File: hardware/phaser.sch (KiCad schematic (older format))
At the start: 38 parts, among them IC1 STM32F042K4U6, IC2 MCP1700, P1 CONN_01X03, P2 SWD_TC, T1 230/6+6 1VA, U1 VTX-214-003-105

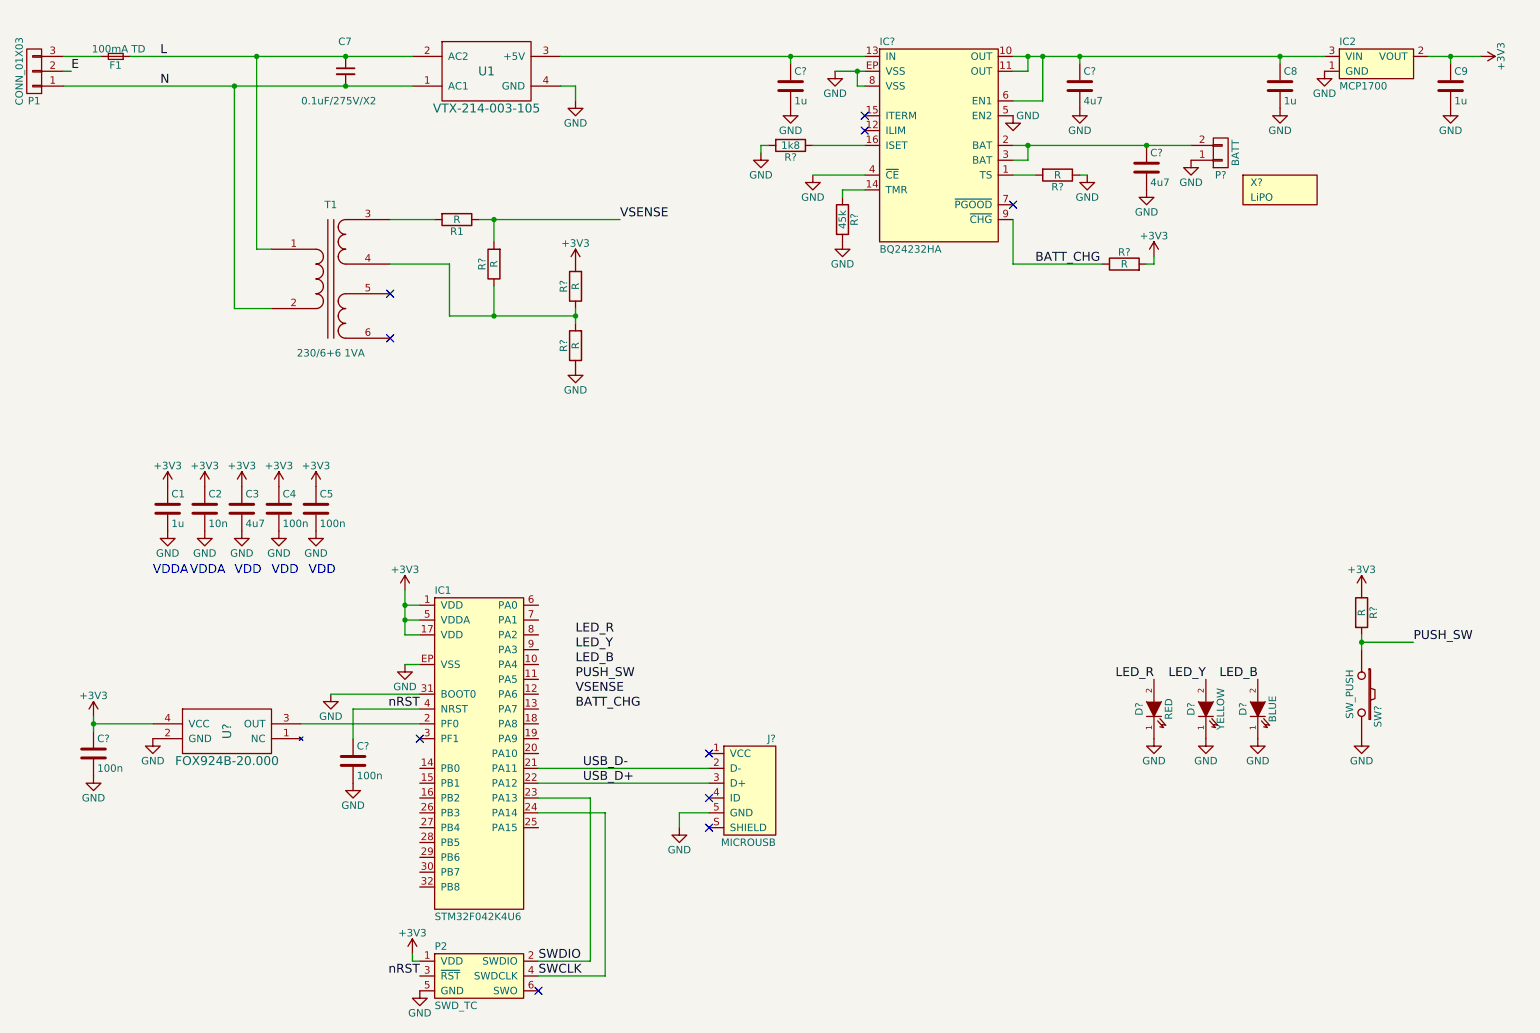
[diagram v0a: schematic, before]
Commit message: part selection
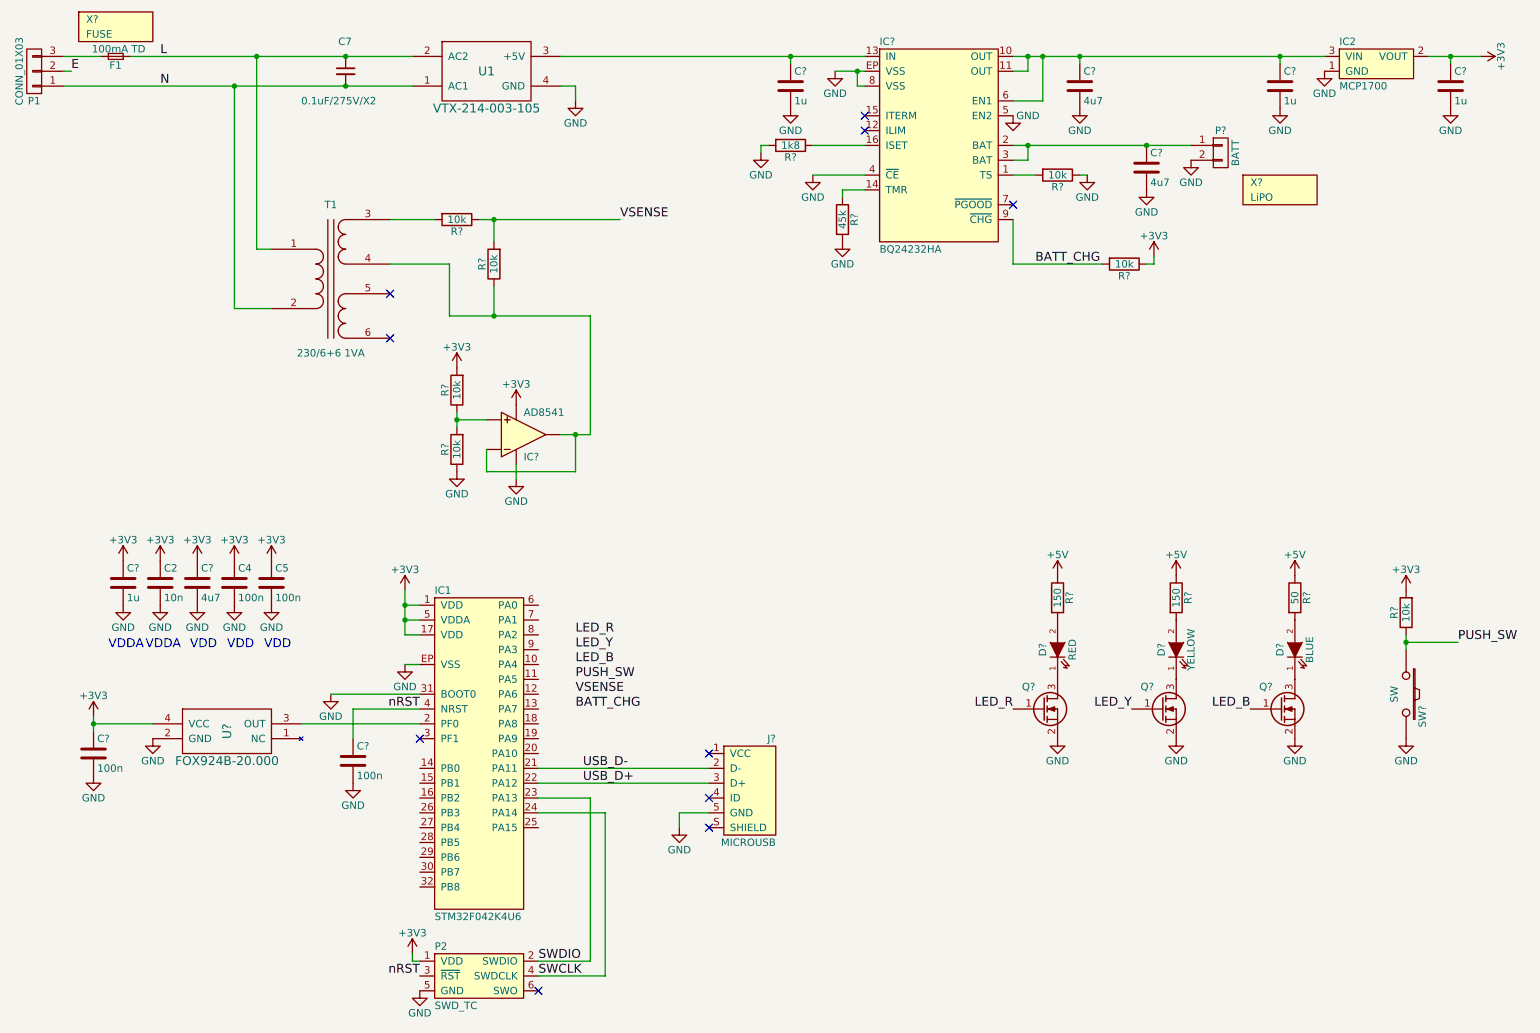
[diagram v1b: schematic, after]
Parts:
- removed C1, C8, C9: 1u, agg:0603, symbol C
- removed C3, C?: 4u7, agg:0603, symbol C
- removed C?: 100n, agg:0603, symbol C
- removed R1, R? (x3): R, agg:0603, symbol R
- removed R? (x2): R, symbol R
- added C?: 100n, agg:0603, symbol C
- added C? (x3): 1u, agg:0603, symbol C
- added C? (x2): 4u7, agg:0603, symbol C
- added IC?: AD8541, agg:SOT-23-5, symbol AD8541
- added Q? (x3): BSS138P, agg:SOT-23, symbol Q_NMOS_GSD
- added R? (x6): 10k, agg:0603, symbol R
- added R? (x2): 150, agg:0603, symbol R
- added R?: 50, agg:0603, symbol R
- added X?: FUSE, symbol PART
- C2: Farnell (none) -> 2496828
- C7: Farnell (none) -> 1198295
- C?: footprint (none) -> agg:0603; Farnell (none) -> 9227776
- C?: footprint (none) -> agg:0603; Farnell (none) -> 2496930
- D?: footprint (none) -> agg:SIL-254P-02; Farnell (none) -> 2431256
- D?: footprint (none) -> agg:SIL-254P-02; Farnell (none) -> 2431258
- D?: footprint (none) -> agg:SIL-254P-02; Farnell (none) -> 2431252
- F1: Farnell (none) -> 1162740
- P?: footprint (none) -> Connectors_JST:JST_PH_S2B-PH-K_02x2.00mm_Angled; Farnell (none) -> 9491902
- R?: footprint (none) -> agg:0603; Farnell (none) -> 2059468
- R?: footprint (none) -> agg:0603; Farnell (none) -> 2303162
- R?: value R -> 10k; footprint (none) -> agg:0603; Farnell (none) -> 9238603
- SW?: value SW_PUSH -> SW; footprint (none) -> agg:SIL-254P-02; Farnell (none) -> 1634622
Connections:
- net +3V3: now also C?.1, C?.1, C?.1, C?.1, IC?.5 (V+), R?.1, R?.2, R?.2
- net BATT_CHG: now also R?.2
- net GND: now also P?.2 (P2), C?.2, C?.2, C?.2, C?.2, C?.2, C?.2, IC?.2 (V-), Q?.2 (S), Q?.2 (S), Q?.2 (S), R?.1; no longer D?.1 (K), D?.1 (K), D?.1 (K), P?.1 (P1)
- net LED_B: now also Q?.1 (G); no longer D?.2 (A)
- net LED_R: now also Q?.1 (G); no longer D?.2 (A)
- net LED_Y: now also Q?.1 (G); no longer D?.2 (A)
- net PUSH_SW: now also R?.1
- net VSENSE: now also R?.1, R?.2
- net at T1.3 (SA): now also R?.2
- net at T1.4 (SB): now also IC?.1 (OUT), IC?.4 (-), R?.1
- net at C?.1, IC2.3 (VIN), IC?.10 (OUT)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: now also C?.1
- net at IC?.2 (BAT), IC?.3 (BAT): now also P?.1 (P1), C?.1; no longer P?.2 (P2)
- new net: D?.1 (K), Q?.3 (D) (x3)
- new net: D?.2 (A), R?.2 (x3)
- new net: IC?.3 (+), R?.1, R?.2
- new net +5V: R?.1, R?.1, R?.1
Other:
- moved on the sheet: C2, C4, C5, D?, SW?
